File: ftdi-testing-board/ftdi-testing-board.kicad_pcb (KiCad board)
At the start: 2 copper layers, 55 parts, among them J1 Conn_01x14_Male, J10 Conn_01x04_Male, J11 Conn_01x05_Male, J12 Conn_01x05_Male, J13 Conn_01x05_Male, J2 Conn_01x06_Male, J3 UJ31-CH-G2-SMT-TR, J4 Conn_01x14_Male, J5 Conn_01x10_Male, J6 Conn_01x08_Male, J7 Conn_01x04_Male, J8 Conn_01x05_Male, J9 Conn_01x04_Male, Q1 MMBT2222LT1G, Q2 MMBT2222LT1G, U1 TS5A3153DCUR, U2 TS5A3153DCUR, U3 ESP32-WROOM-32D, U4 4.7uF, U5 AP2115M-3.3TRG1, U6 4.7uF, U7 4.7uF, U8 FT260S-U, U9 FT312D-32L1C-R

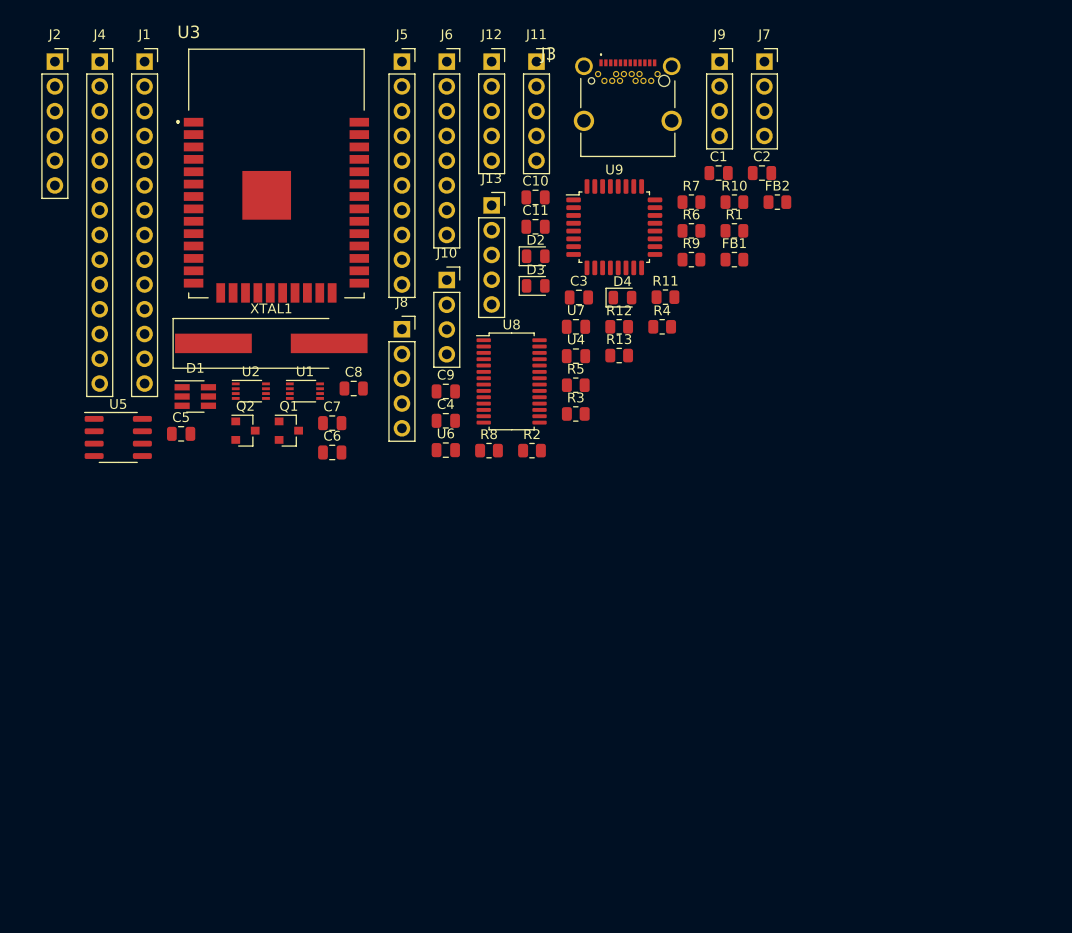
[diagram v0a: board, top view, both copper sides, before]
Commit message: Added Gerber Files, BOM and 3D Model exports
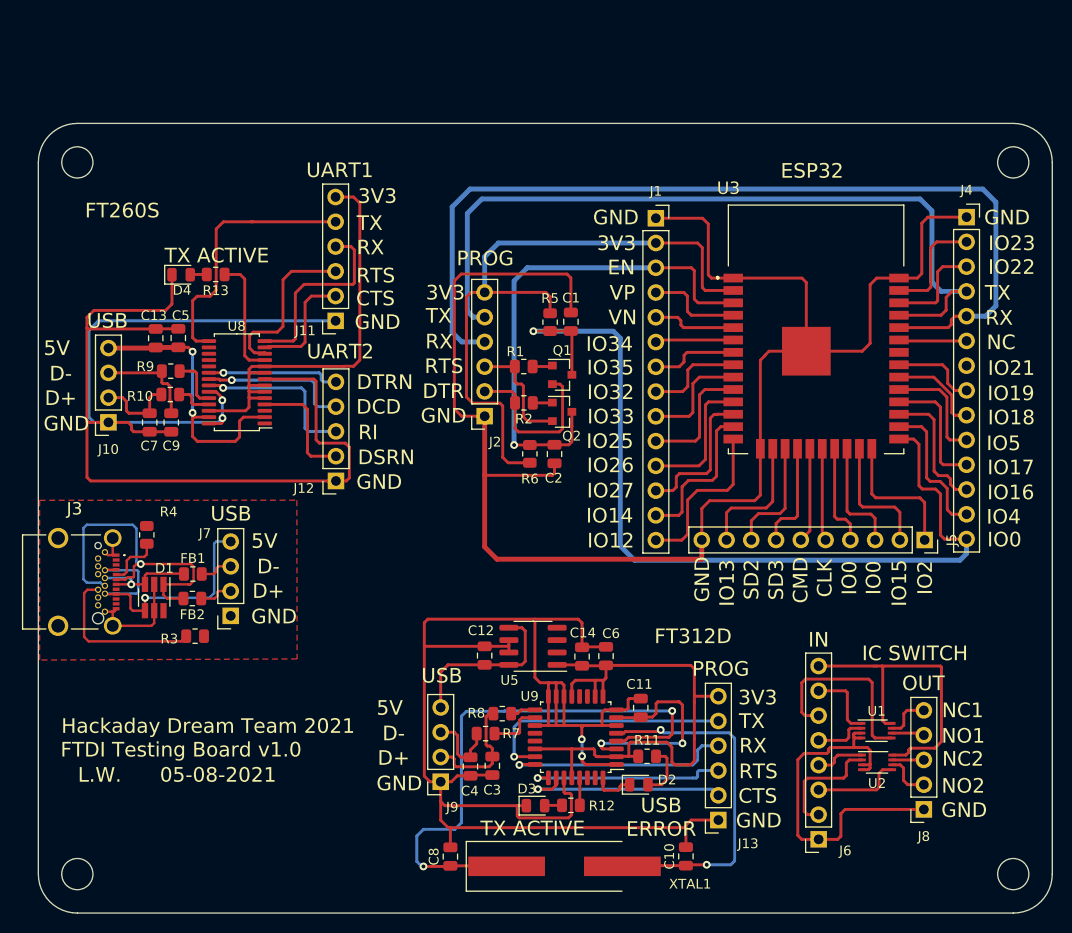
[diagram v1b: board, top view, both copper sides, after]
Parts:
- added REF**: MountingHole_3.2mm_M3, MountingHole:MountingHole_3.2mm_M3, F.Cu at (142.0, 94.0)
- added REF**: MountingHole_3.2mm_M3, MountingHole:MountingHole_3.2mm_M3, F.Cu at (238.0, 94.0)
- added REF**: MountingHole_3.2mm_M3, MountingHole:MountingHole_3.2mm_M3, F.Cu at (238.0, 167.0)
- added REF**: MountingHole_3.2mm_M3, MountingHole:MountingHole_3.2mm_M3, F.Cu at (142.0, 167.0)
- J11, J13: value Conn_01x05_Male -> Conn_01x06_Male; footprint Connector_PinSocket_2.54mm:PinSocket_1x05_P2.54mm_Vertical -> Connector_PinSocket_2.54mm:PinSocket_1x06_P2.54mm_Vertical
- moved J4 90.3 mm to (233.2, 99.6)
- moved J6 88.4 mm to (218.0, 163.4), turned to 180 degrees
- moved J9 79.2 mm to (179.3, 157.5), turned to 180 degrees
- moved J7 78.9 mm to (157.7, 140.5), turned to 180 degrees
- moved J3 75.2 mm to (140.0, 137.0), turned to 270 degrees
- moved U2 74.7 mm to (224.0, 155.5)
- moved J8 72.7 mm to (228.8, 160.4), turned to 180 degrees
- moved J5 72.7 mm to (228.9, 132.7), turned to 270 degrees
- moved FB2 72.5 mm to (153.8, 138.7), turned to 180 degrees
- moved C10 69.3 mm to (204.4, 165.2), turned to 90 degrees
- moved U1 68.2 mm to (224.0, 152.3)
- moved J13 67.2 mm to (207.8, 161.5), turned to 180 degrees
- moved FB1 64.2 mm to (153.8, 136.2), turned to 180 degrees
- moved XTAL1 61.5 mm to (192.0, 166.2)
- moved R10 61.1 mm to (151.5, 117.8), turned to 180 degrees
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- renumbered U4 to C12, U6 to C13, U7 to C14
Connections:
- C14 pad 1: Net-(C6-Pad1) -> Net-(C14-Pad1)
- C6 pad 1: Net-(C6-Pad1) -> Net-(C14-Pad1)
- R11 pad 1: Net-(C6-Pad1) -> Net-(C14-Pad1)
- U5 pad 1: Net-(C6-Pad1) -> Net-(C14-Pad1)
- U8 pad 10: Net-(U8-Pad10) -> 3V3_FT260
- U8 pad 26: Net-(U8-Pad10) -> 3V3_FT260
- U8 pad 5: Net-(U8-Pad10) -> 3V3_FT260
- U8 pad 6: Net-(U8-Pad10) -> 3V3_FT260
- U8 pad 7: Net-(U8-Pad10) -> 3V3_FT260
- U8 pad 9: Net-(U8-Pad10) -> 3V3_FT260
- U9 pad 10: Net-(C6-Pad1) -> Net-(C14-Pad1)
- U9 pad 13: Net-(C6-Pad1) -> Net-(C14-Pad1)
- U9 pad 2: Net-(C6-Pad1) -> Net-(C14-Pad1)
- U9 pad 22: Net-(C6-Pad1) -> Net-(C14-Pad1)
- U9 pad 28: Net-(C6-Pad1) -> Net-(C14-Pad1)
- U9 pad 8: GND1 -> GND2
- U9 pad 9: Net-(C6-Pad1) -> Net-(C14-Pad1)
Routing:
- net GND: track 0.00 -> 164.7 mm
- net GND2: track 0.00 -> 156.6 mm, vias 0 -> 2
- net GND3: track 0.00 -> 147.1 mm, vias 0 -> 2
- net ESP_RX: track 0.00 -> 95.5 mm
- net ESP_IO0: track 0.00 -> 93.0 mm, vias 0 -> 1
- net ESP_TX: track 0.00 -> 80.8 mm
- net +3V3: track 0.00 -> 67.5 mm
- net Net-(C14-Pad1): track 0.00 -> 60.4 mm
- net Net-(C8-Pad1): track 0.00 -> 58.5 mm, vias 0 -> 2
- net ESP_EN: track 0.00 -> 52.2 mm, vias 0 -> 1
- net 3V3_FT260: track 0.00 -> 45.3 mm
- net GNDA: track 0.00 -> 38.4 mm
- net Net-(C10-Pad1): track 0.00 -> 37.1 mm, vias 0 -> 2
- net Net-(D1-Pad1): track 0.00 -> 34.7 mm, vias 0 -> 1
- net Net-(J6-Pad8): track 0.00 -> 32.7 mm
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- added copper zone on F.Cu, net GND1
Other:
- board outline added: 104 x 81 mm
- rule via_min_size: 0.4 -> 0.2
- board text added: "3V3"
- board text added: "5V"
- board text added: "CLK"
- board text added: "CMD"
- board text added: "CTS"
- board text added: "D+"
- board text added: "D-"
- board text added: "DCD"
- board text added: "DSRN"
- board text added: "DTR"
- board text added: "DTRN"
- board text added: "EN"
- board text added: "ESP32"
- board text added: "FT260S"
- board text added: "FT312D"
- board text added: "FTDI Testing Board v1.0"
- board text added: "GND"
- board text added: "Hackaday Dream Team 2021"
- board text added: "IC SWITCH"
- board text added: "IN"
- board text added: "IO0"
- board text added: "IO12"
- board text added: "IO13"
- board text added: "IO14"
- board text added: "IO15"
- board text added: "IO16"
- board text added: "IO17"
- board text added: "IO18"
- board text added: "IO19"
- board text added: "IO2"
- board text added: "IO21"
- board text added: "IO22"
- board text added: "IO23"
- board text added: "IO25"
- board text added: "IO26"
- board text added: "IO27"
- board text added: "IO32"
- board text added: "IO33"
- board text added: "IO34"
- board text added: "IO35"
- board text added: "IO4"
- board text added: "IO5"
- board text added: "L.W. 05-08-2021"
- board text added: "NC"
- board text added: "NC1"
- board text added: "NC2"
- board text added: "NO1"
- board text added: "NO2"
- board text added: "OUT"
- board text added: "PROG"
- board text added: "RI"
- board text added: "RTS"
- board text added: "RX"
- board text added: "SD2"
- board text added: "SD3"
- board text added: "TX"
- board text added: "TX ACTIVE"
- board text added: "UART1"
- board text added: "UART2"
- board text added: "USB"
- board text added: "USB ERROR"
- board text added: "VN"
- board text added: "VP"
